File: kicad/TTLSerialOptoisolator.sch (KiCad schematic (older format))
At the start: 8 parts, among them P1 CONN_4, P2 CONN_4, U1 817C, U2 817C

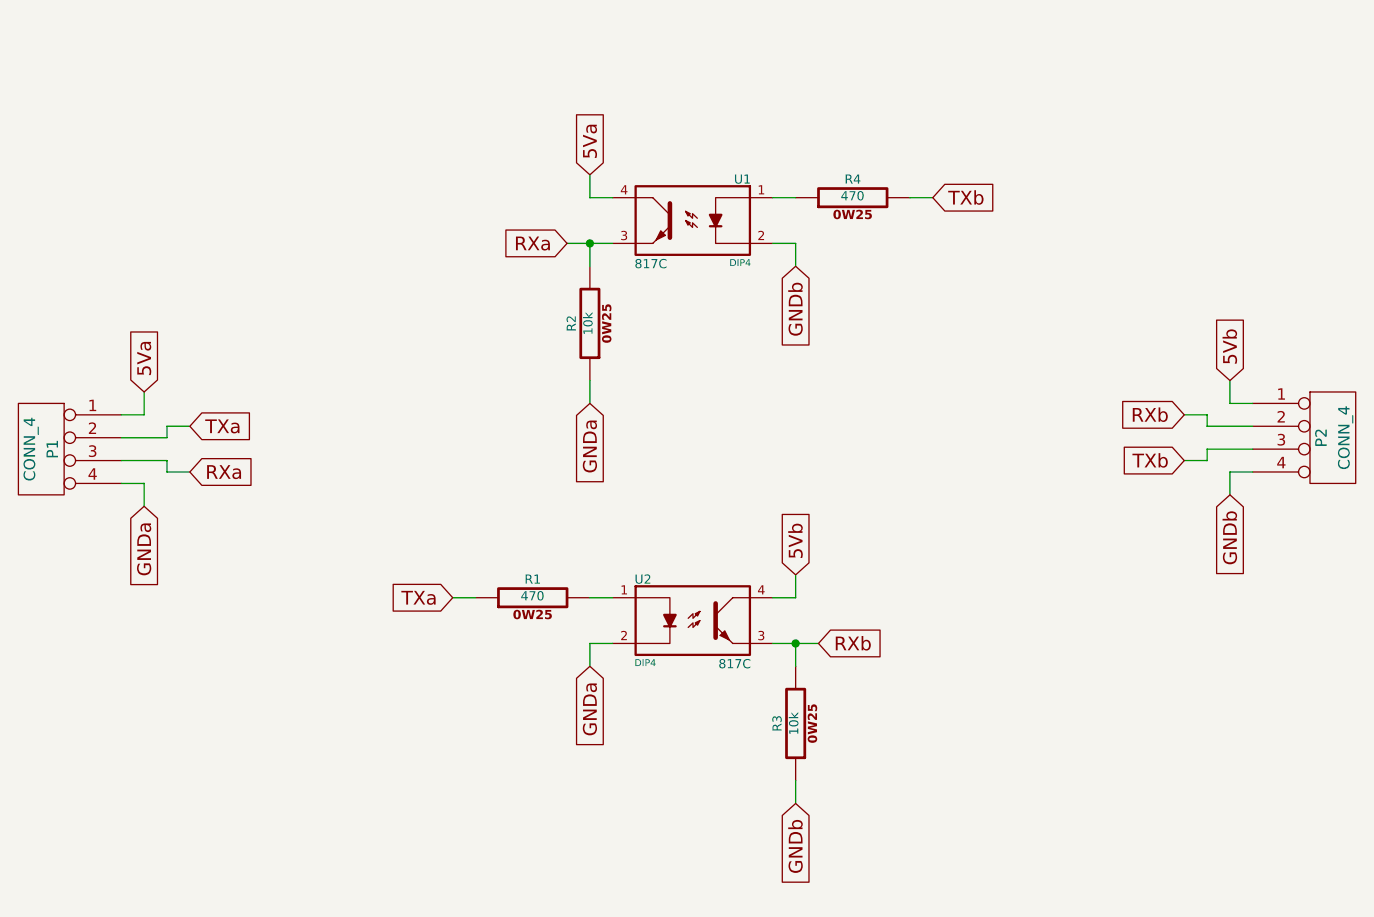
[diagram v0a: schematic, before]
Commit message: iterating on board layout
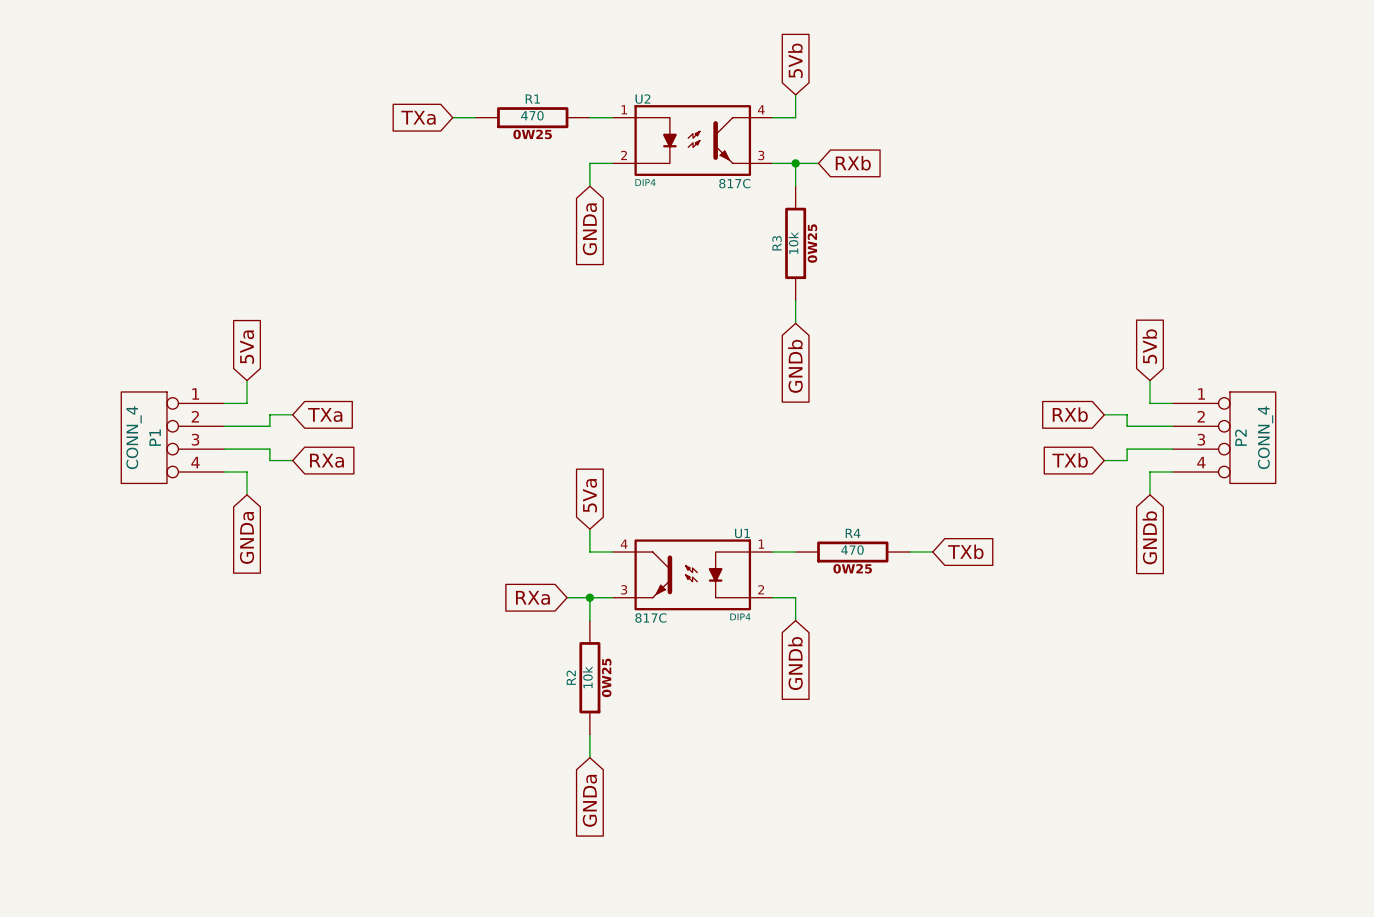
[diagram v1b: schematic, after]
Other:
- moved on the sheet: P1, P2, R1, R2, R3, R4, U1, U2
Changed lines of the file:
@@
 L 817C U2
 U 1 1 552955FE
-P 5250 4450
-F 0 "U2" H 4995 4630 40  0000 L CNN
-F 1 "817C" H 5505 4260 40  0000 R CNN
-F 2 "DIP4" H 4995 4265 30  0000 L CNN
-F 3 "~" H 5250 4450 60  0000 C CNN
-	1    5250 4450
+P 5250 2350
+F 0 "U2" H 4995 2530 40  0000 L CNN
+F 1 "817C" H 5505 2160 40  0000 R CNN
+F 2 "DIP4" H 4995 2165 30  0000 L CNN
+F 3 "~" H 5250 2350 60  0000 C CNN
+	1    5250 2350
 	1    0    0    -1
 $EndComp
@@
 L 817C U1
 U 1 1 5529567E
-P 5250 2700
-F 0 "U1" H 4995 2880 40  0000 L CNN
-F 1 "817C" H 5505 2510 40  0000 R CNN
-F 2 "DIP4" H 4995 2515 30  0000 L CNN
-F 3 "~" H 5250 2700 60  0000 C CNN
-	1    5250 2700
+P 5250 4250
+F 0 "U1" H 4995 4430 40  0000 L CNN
+F 1 "817C" H 5505 4060 40  0000 R CNN
+F 2 "DIP4" H 4995 4065 30  0000 L CNN
+F 3 "~" H 5250 4250 60  0000 C CNN
+	1    5250 4250
 	-1   0    0    -1
 $EndComp
@@
 L CONN_4 P1
 U 1 1 552956C5
-P 2400 3700
-F 0 "P1" V 2350 3700 50  0000 C CNN
-F 1 "CONN_4" V 2450 3700 50  0000 C CNN
-F 2 "" H 2400 3700 60  0000 C CNN
-F 3 "" H 2400 3700 60  0000 C CNN
-	1    2400 3700
+P 2850 3650
+F 0 "P1" V 2800 3650 50  0000 C CNN
+F 1 "CONN_4" V 2900 3650 50  0000 C CNN
+F 2 "" H 2850 3650 60  0000 C CNN
+F 3 "" H 2850 3650 60  0000 C CNN
+	1    2850 3650
 	-1   0    0    -1
 $EndComp
-Text GLabel 2850 3450 1    60   Input ~ 0
+Text GLabel 3300 3400 1    60   Input ~ 0
 5Va
-Text GLabel 2850 3950 3    60   Input ~ 0
+Text GLabel 3300 3900 3    60   Input ~ 0
 GNDa
-Text GLabel 3050 3800 2    60   Input ~ 0
+Text GLabel 3500 3750 2    60   Input ~ 0
 RXa
-Text GLabel 3050 3600 2    60   Input ~ 0
+Text GLabel 3500 3550 2    60   Input ~ 0
 TXa
 Wire Wire Line
-	2750 3550 2850 3550
-Wire Wire Line
-	2850 3550 2850 3450
-Wire Wire Line
-	2750 3850 2850 3850
-Wire Wire Line
-	2850 3850 2850 3950
-Wire Wire Line
-	2750 3750 2950 3750
-Wire Wire Line
-	2950 3750 2950 3800
-Wire Wire Line
-	2950 3800 3050 3800
-Wire Wire Line
-	2750 3650 2950 3650
-Wire Wire Line
-	2950 3650 2950 3600
-Wire Wire Line
-	2950 3600 3050 3600
+	3200 3500 3300 3500
+Wire Wire Line
+	3300 3500 3300 3400
+Wire Wire Line
+	3200 3800 3300 3800
+Wire Wire Line
+	3300 3800 3300 3900
+Wire Wire Line
+	3200 3700 3400 3700
+Wire Wire Line
+	3400 3700 3400 3750
+Wire Wire Line
+	3400 3750 3500 3750
+Wire Wire Line
+	3200 3600 3400 3600
+Wire Wire Line
+	3400 3600 3400 3550
+Wire Wire Line
+	3400 3550 3500 3550
 $Comp
 L R_0W25 R1
 U 1 1 5529585F
-P 4550 4350
-F 0 "R1" V 4630 4350 40  0000 C CNN
-F 1 "470" V 4557 4351 40  0000 C CNN
-F 2 "~" V 4480 4350 30  0000 C CNN
-F 3 "~" H 4550 4350 30  0000 C CNN
-	1    4550 4350
+P 4550 2250
+F 0 "R1" V 4630 2250 40  0000 C CNN
+F 1 "470" V 4557 2251 40  0000 C CNN
+F 2 "~" V 4480 2250 30  0000 C CNN
+F 3 "~" H 4550 2250 30  0000 C CNN
+	1    4550 2250
 	0    -1   -1   0
 $EndComp
-Text GLabel 4800 4650 3    60   Input ~ 0
+Text GLabel 4800 2550 3    60   Input ~ 0
 GNDa
 Wire Wire Line
-	4900 4550 4800 4550
-Wire Wire Line
-	4800 4550 4800 4650
-Wire Wire Line
-	4800 4350 4900 4350
-Text GLabel 4200 4350 0    60   Input ~ 0
+	4900 2450 4800 2450
+Wire Wire Line
+	4800 2450 4800 2550
+Wire Wire Line
+	4800 2250 4900 2250
+Text GLabel 4200 2250 0    60   Input ~ 0
 TXa
 Wire Wire Line
-	4200 4350 4300 4350
+	4200 2250 4300 2250
 $Comp
 L CONN_4 P2
 U 1 1 552958B7
-P 8050 3650
-F 0 "P2" V 8000 3650 50  0000 C CNN
-F 1 "CONN_4" V 8100 3650 50  0000 C CNN
-F 2 "" H 8050 3650 60  0000 C CNN
-F 3 "" H 8050 3650 60  0000 C CNN
-	1    8050 3650
+P 7700 3650
+F 0 "P2" V 7650 3650 50  0000 C CNN
+F 1 "CONN_4" V 7750 3650 50  0000 C CNN
+F 2 "" H 7700 3650 60  0000 C CNN
+F 3 "" H 7700 3650 60  0000 C CNN
+	1    7700 3650
 	1    0    0    -1
 $EndComp
-Text GLabel 7600 3400 1    60   Input ~ 0
+Text GLabel 7250 3400 1    60   Input ~ 0
 5Vb
-Text GLabel 7600 3900 3    60   Input ~ 0
+Text GLabel 7250 3900 3    60   Input ~ 0
 GNDb
-Text GLabel 7400 3550 0    60   Input ~ 0
+Text GLabel 7050 3550 0    60   Input ~ 0
 RXb
-Text GLabel 7400 3750 0    60   Input ~ 0
+Text GLabel 7050 3750 0    60   Input ~ 0
 TXb
 Wire Wire Line
-	7700 3500 7600 3500
-Wire Wire Line
-	7600 3500 7600 3400
-Wire Wire Line
-	7700 3800 7600 3800
-Wire Wire Line
-	7600 3800 7600 3900
-Wire Wire Line
-	7700 3700 7500 3700
-Wire Wire Line
-	7500 3700 7500 3750
-Wire Wire Line
-	7500 3750 7400 3750
-Wire Wire Line
-	7700 3600 7500 3600
-Wire Wire Line
-	7500 3600 7500 3550
-Wire Wire Line
-	7500 3550 7400 3550
+	7350 3500 7250 3500
+Wire Wire Line
+	7250 3500 7250 3400
+Wire Wire Line
+	7350 3800 7250 3800
+Wire Wire Line
+	7250 3800 7250 3900
+Wire Wire Line
+	7350 3700 7150 3700
+Wire Wire Line
+	7150 3700 7150 3750
+Wire Wire Line
+	7150 3750 7050 3750
+Wire Wire Line
+	7350 3600 7150 3600
+Wire Wire Line
+	7150 3600 7150 3550
+Wire Wire Line
+	7150 3550 7050 3550
 $Comp
 L R_0W25 R4
 U 1 1 552958D6
-P 5950 2600
-F 0 "R4" V 6030 2600 40  0000 C CNN
-F 1 "470" V 5957 2601 40  0000 C CNN
-F 2 "~" V 5880 2600 30  0000 C CNN
-F 3 "~" H 5950 2600 30  0000 C CNN
-	1    5950 2600
+P 5950 4150
+F 0 "R4" V 6030 4150 40  0000 C CNN
+F 1 "470" V 5957 4151 40  0000 C CNN
+F 2 "~" V 5880 4150 30  0000 C CNN
+F 3 "~" H 5950 4150 30  0000 C CNN
+	1    5950 4150
 	0    -1   -1   0
 $EndComp
-Text GLabel 6300 2600 2    60   Input ~ 0
+Text GLabel 6300 4150 2    60   Input ~ 0
 TXb
-Text GLabel 5700 2900 3    60   Input ~ 0
+Text GLabel 5700 4450 3    60   Input ~ 0
 GNDb
 Wire Wire Line
-	5600 2800 5700 2800
-Wire Wire Line
-	5700 2800 5700 2900
-Wire Wire Line
-	5600 2600 5700 2600
-Wire Wire Line
-	6200 2600 6300 2600
+	5600 4350 5700 4350
+Wire Wire Line
+	5700 4350 5700 4450
+Wire Wire Line
+	5600 4150 5700 4150
+Wire Wire Line
+	6200 4150 6300 4150
 $Comp
 L R_0W25 R2
 U 1 1 55295938
-P 4800 3150
-F 0 "R2" V 4880 3150 40  0000 C CNN
-F 1 "10k" V 4807 3151 40  0000 C CNN
-F 2 "~" V 4730 3150 30  0000 C CNN
-F 3 "~" H 4800 3150 30  0000 C CNN
-	1    4800 3150
+P 4800 4700
+F 0 "R2" V 4880 4700 40  0000 C CNN
+F 1 "10k" V 4807 4701 40  0000 C CNN
+F 2 "~" V 4730 4700 30  0000 C CNN
+F 3 "~" H 4800 4700 30  0000 C CNN
+	1    4800 4700
 	-1   0    0    1
 $EndComp
-Text GLabel 4800 2500 1    60   Input ~ 0
+Text GLabel 4800 4050 1    60   Input ~ 0
 5Va
 Wire Wire Line
-	4800 2500 4800 2600
-Wire Wire Line
-	4800 2600 4900 2600
-Wire Wire Line
-	4700 2800 4900 2800
-Wire Wire Line
-	4800 2800 4800 2900
-Text GLabel 4800 3500 3    60   Input ~ 0
+	4800 4050 4800 4150
+Wire Wire Line
+	4800 4150 4900 4150
+Wire Wire Line
+	4700 4350 4900 4350
+Wire Wire Line
+	4800 4350 4800 4450
+Text GLabel 4800 5050 3    60   Input ~ 0
 GNDa
 Wire Wire Line
-	4800 3400 4800 3500
-Text GLabel 4700 2800 0    60   Input ~ 0
+	4800 4950 4800 5050
+Text GLabel 4700 4350 0    60   Input ~ 0
 RXa
-Connection ~ 4800 2800
+Connection ~ 4800 4350
 $Comp
 L R_0W25 R3
 U 1 1 552959CF
-P 5700 4900
-F 0 "R3" V 5780 4900 40  0000 C CNN
-F 1 "10k" V 5707 4901 40  0000 C CNN
-F 2 "~" V 5630 4900 30  0000 C CNN
-F 3 "~" H 5700 4900 30  0000 C CNN
-	1    5700 4900
+P 5700 2800
+F 0 "R3" V 5780 2800 40  0000 C CNN
+F 1 "10k" V 5707 2801 40  0000 C CNN
+F 2 "~" V 5630 2800 30  0000 C CNN
+F 3 "~" H 5700 2800 30  0000 C CNN
+	1    5700 2800
 	-1   0    0    1
 $EndComp
-Text GLabel 5700 4250 1    60   Input ~ 0
+Text GLabel 5700 2150 1    60   Input ~ 0
 5Vb
-Text GLabel 5700 5250 3    60   Input ~ 0
+Text GLabel 5700 3150 3    60   Input ~ 0
 GNDb
 Wire Wire Line
-	5700 5150 5700 5250
-Wire Wire Line
-	5600 4350 5700 4350
-Wire Wire Line
-	5700 4350 5700 4250
-Wire Wire Line
-	5600 4550 5800 4550
-Wire Wire Line
-	5700 4550 5700 4650
-Text GLabel 5800 4550 2    60   Input ~ 0
+	5700 3050 5700 3150
+Wire Wire Line
+	5600 2250 5700 2250
+Wire Wire Line
+	5700 2250 5700 2150
+Wire Wire Line
+	5600 2450 5800 2450
+Wire Wire Line
+	5700 2450 5700 2550
+Text GLabel 5800 2450 2    60   Input ~ 0
 RXb
-Connection ~ 5700 4550
+Connection ~ 5700 2450
 $EndSCHEMATC
